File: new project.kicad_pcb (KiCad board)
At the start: 2 copper layers, 33.8 x 23 mm, 4 parts, among them J1 LED 0.170amps, J2 Tractive Battery

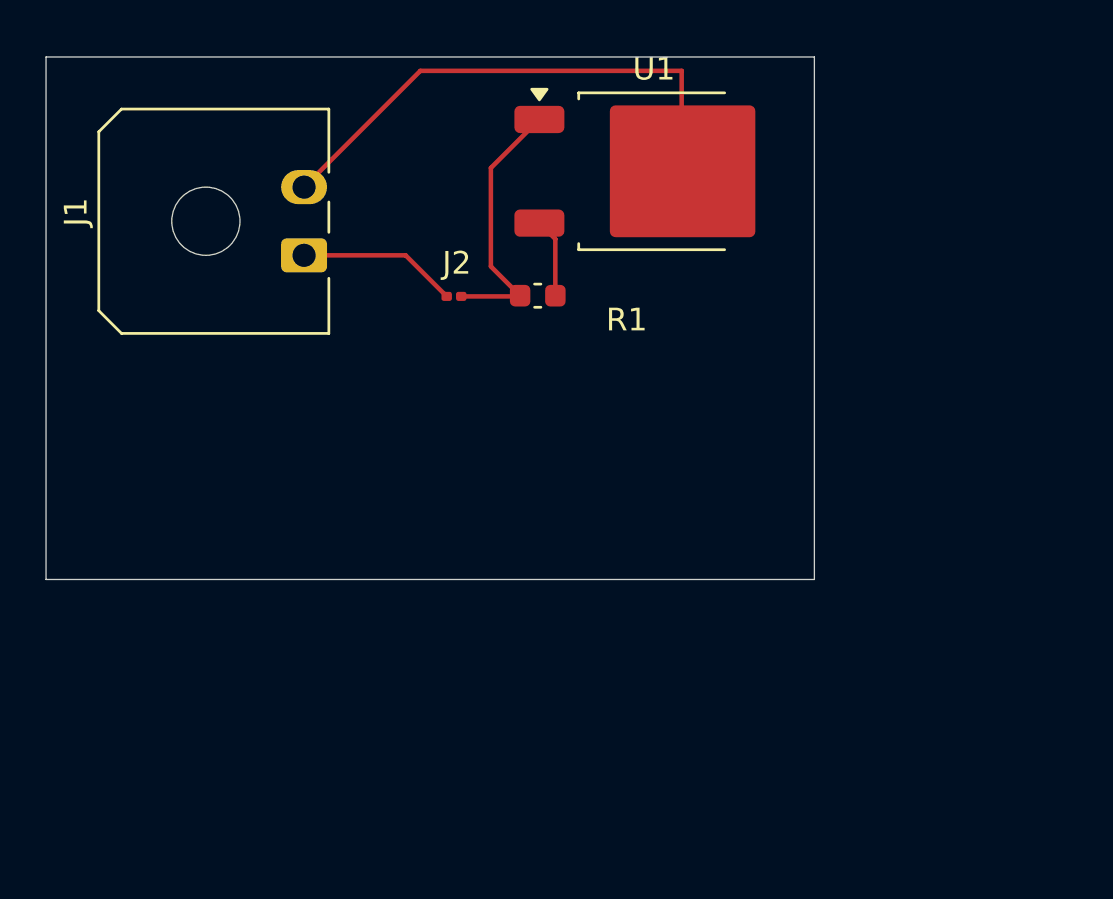
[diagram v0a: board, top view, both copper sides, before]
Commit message: Finally fixed
Please upload the changes
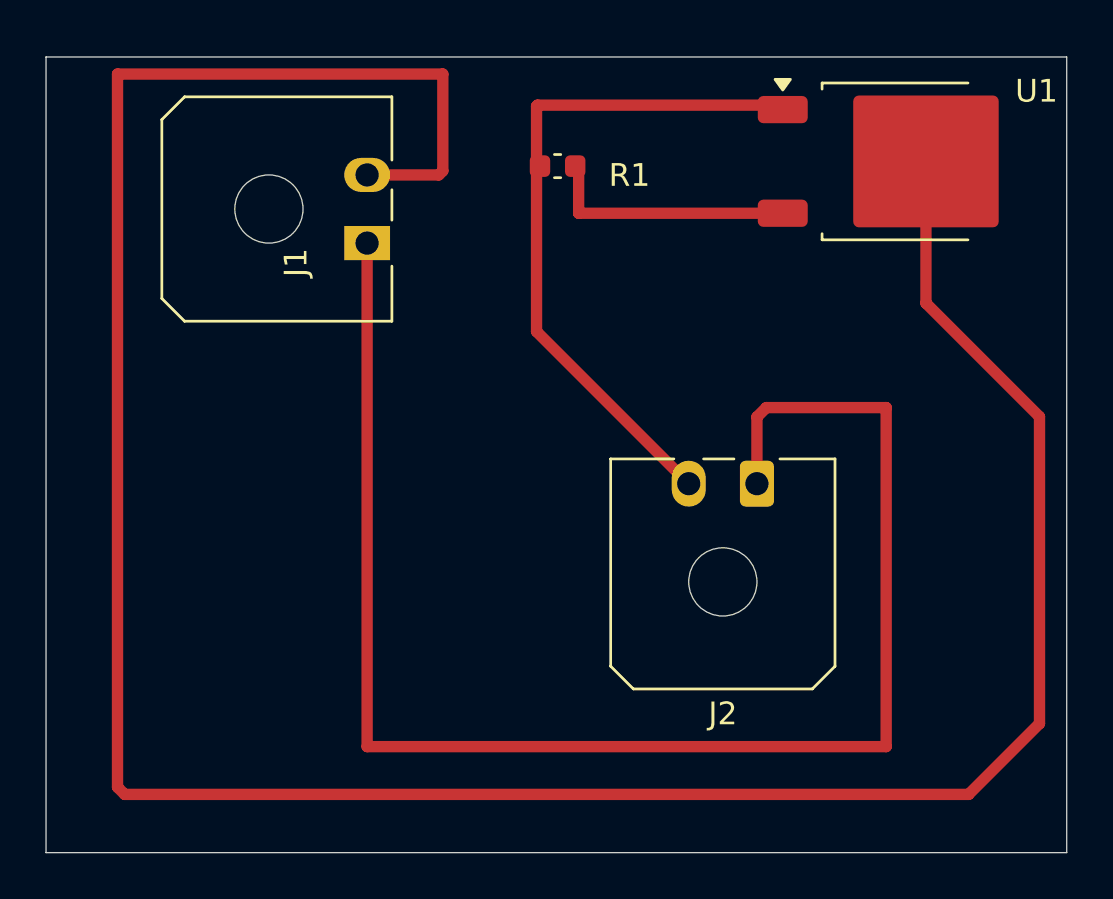
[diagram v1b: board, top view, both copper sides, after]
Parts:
- J2: footprint Resistor_SMD:R_0201_0603Metric -> Connector_Molex:Molex_Micro-Fit_3.0_43650-0200_1x02_P3.00mm_Horizontal
- R1: value 1800 -> 18000
- moved J2 15.7 mm to (135.5, 77.4), turned to 180 degrees
- moved U1 10.7 mm to (141.6, 63.3)
- moved R1 5.77 mm to (126.7, 63.5)
- moved J1 2.82 mm to (118.3, 66.9)
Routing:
- net Net-(J1-Pin_2): track 23.2 -> 122.2 mm
- net +4V: track 7.02 -> 68.7 mm
- net GND: track 11.8 -> 30.4 mm
- net Net-(U1-Cathode): track 3.48 -> 10.9 mm
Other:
- board size 33.8 x 23 mm -> 44.9 x 35 mm
